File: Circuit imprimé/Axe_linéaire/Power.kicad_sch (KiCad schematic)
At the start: 6 parts, among them Q2 LP2301LT1G

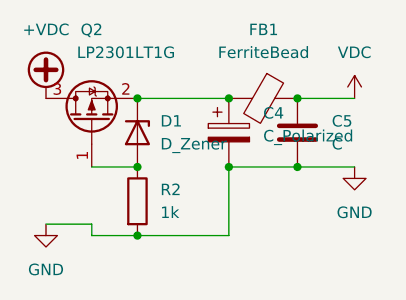
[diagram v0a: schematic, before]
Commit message: circuit V1
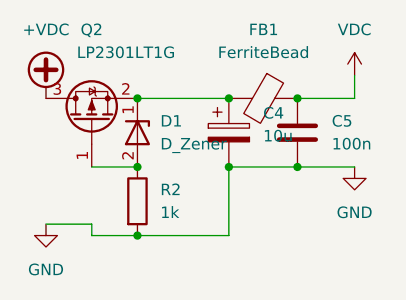
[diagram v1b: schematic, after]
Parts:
- C4: value C_Polarized -> 10u; footprint (none) -> Capacitor_SMD:CP_Elec_6.3x7.7
- C5: value C -> 100n; footprint (none) -> Library:Cap 100nf 0805
- D1: footprint (none) -> Library:SOD223
- FB1: footprint (none) -> Library:ferrite Bead
- R2: footprint (none) -> Resistor_SMD:R_0603_1608Metric
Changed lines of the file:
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@@
+    (stroke (width 0) (type default) (color 0 0 0 0))
+  )
+  (wire (pts (xy 66.04 20.32) (xy 66.04 22.86))
     (stroke (width 0) (type default) (color 0 0 0 0))
   )
@@
       (effects (font (size 1.27 1.27)) (justify left))
     )
-    (property "Value" "C_Polarized" (id 1) (at 55.88 27.0509 0)
+    (property "Value" "10u" (id 1) (at 55.88 27.0509 0)
       (effects (font (size 1.27 1.27)) (justify left))
     )
-    (property "Footprint" "" (id 2) (at 53.0352 30.48 0)
+    (property "Footprint" "Capacitor_SMD:CP_Elec_6.3x7.7" (id 2) (at 53.0352 30.48 0)
       (effects (font (size 1.27 1.27)) hide)
     )
@@
     (property "Reference" "FB1" (id 0) (at 55.9308 15.24 90))
     (property "Value" "FerriteBead" (id 1) (at 55.9308 17.78 90))
-    (property "Footprint" "" (id 2) (at 55.88 21.082 90)
+    (property "Footprint" "Library:ferrite Bead" (id 2) (at 55.88 21.082 90)
       (effects (font (size 1.27 1.27)) hide)
     )
@@
       (effects (font (size 1.27 1.27)) (justify left))
     )
-    (property "Footprint" "" (id 2) (at 41.91 26.67 0)
+    (property "Footprint" "Library:SOD223" (id 2) (at 41.91 26.67 0)
       (effects (font (size 1.27 1.27)) hide)
     )
@@
     (pin "1")
   )
-  (symbol (lib_id "power:VDC") (at 66.04 22.86 0) (unit 1)
-    (in_bom yes) (on_board yes) (fields_autoplaced)
-    (property "Reference" "#PWR028" (id 0) (at 66.04 25.4 0)
-      (effects (font (size 1.27 1.27)) hide)
-    )
-    (property "Value" "VDC" (id 1) (at 66.04 17.78 0))
-    (property "Footprint" "" (id 2) (at 66.04 22.86 0)
-      (effects (font (size 1.27 1.27)) hide)
-    )
-    (property "Datasheet" "" (id 3) (at 66.04 22.86 0)
-      (effects (font (size 1.27 1.27)) hide)
-    )
-    (pin "1")
-  )
   (symbol (lib_id "Device:C") (at 59.69 26.67 0) (unit 1)
     (in_bom yes) (on_board yes) (fields_autoplaced)
@@
       (effects (font (size 1.27 1.27)) (justify left))
     )
-    (property "Value" "C" (id 1) (at 63.5 27.9399 0)
+    (property "Value" "100n" (id 1) (at 63.5 27.9399 0)
       (effects (font (size 1.27 1.27)) (justify left))
     )
-    (property "Footprint" "" (id 2) (at 60.6552 30.48 0)
+    (property "Footprint" "Library:Cap 100nf 0805" (id 2) (at 60.6552 30.48 0)
       (effects (font (size 1.27 1.27)) hide)
     )
@@
     (pin "1")
     (pin "2")
+  )
+  (symbol (lib_id "power:VDC") (at 66.04 20.32 0) (unit 1)
+    (in_bom yes) (on_board yes) (fields_autoplaced)
+    (property "Reference" "#PWR0112" (id 0) (at 66.04 22.86 0)
+      (effects (font (size 1.27 1.27)) hide)
+    )
+    (property "Value" "VDC" (id 1) (at 66.04 15.24 0))
+    (property "Footprint" "" (id 2) (at 66.04 20.32 0)
+      (effects (font (size 1.27 1.27)) hide)
+    )
+    (property "Datasheet" "" (id 3) (at 66.04 20.32 0)
+      (effects (font (size 1.27 1.27)) hide)
+    )
+    (pin "1")
   )
   (symbol (lib_id "Transistor_FET:VP0610T") (at 36.83 25.4 90) (unit 1)
@@
       (effects (font (size 1.27 1.27)) (justify left))
     )
-    (property "Footprint" "" (id 2) (at 40.132 34.29 90)
+    (property "Footprint" "Resistor_SMD:R_0603_1608Metric" (id 2) (at 40.132 34.29 90)
       (effects (font (size 1.27 1.27)) hide)
     )
